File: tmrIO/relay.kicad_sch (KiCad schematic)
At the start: 5 parts, among them J1 Screw_Terminal_01x03, K1 Relay_SPDT, Q1 MMBT3904

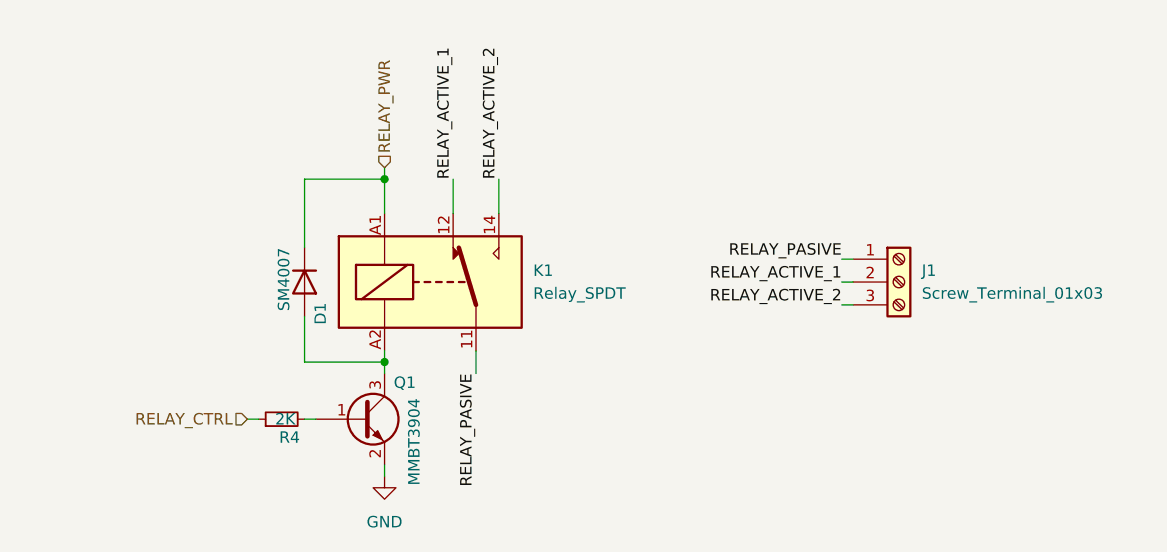
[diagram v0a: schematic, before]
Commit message: tmrIO update
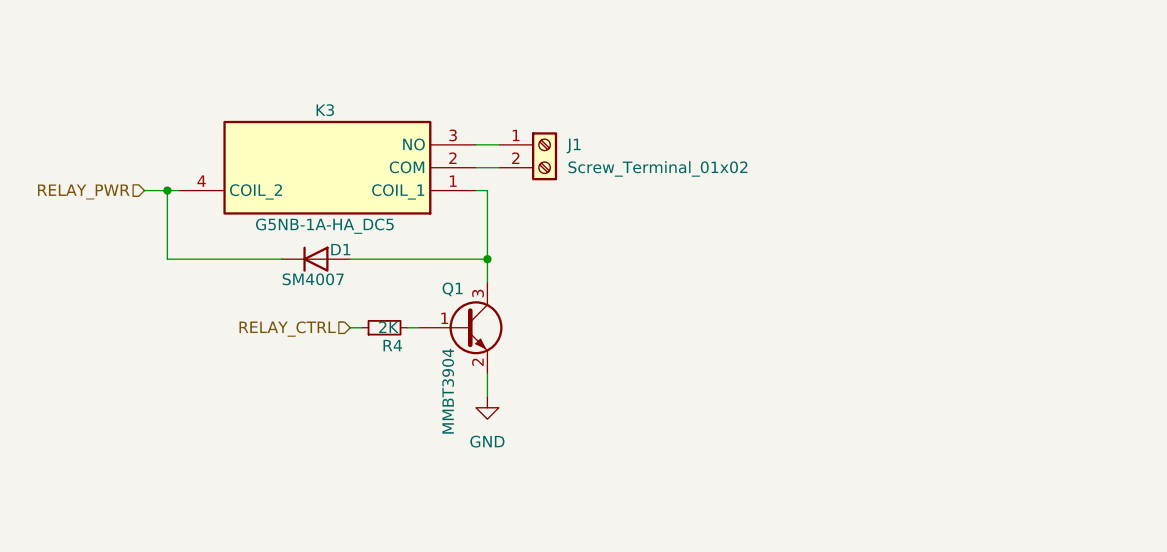
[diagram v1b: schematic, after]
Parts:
- removed J1: Screw_Terminal_01x03, symbol Connector:Screw_Terminal_01x03
- removed K1: Relay_SPDT, symbol Relay:Relay_SPDT
- added J1: Screw_Terminal_01x02, TerminalBlock_Phoenix:TerminalBlock_Phoenix_PT-1,5-2-3.5-H_1x02_P3.50mm_Horizontal, symbol Connector:Screw_Terminal_01x02
- added K3: G5NB-1A-HA_DC5, G5NB-1A-HA:G5NB1AHADC5, symbol G5NB-1A-HA_DC5:G5NB-1A-HA_DC5
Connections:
- net RELAY_PWR: now also K3.4 (COIL_2)
- net at D1.2 (A), Q1.3 (C): now also K3.1 (COIL_1)
- new net: J1.1 (Pin_1), K3.3 (NO)
- new net: J1.2 (Pin_2), K3.2 (COM)
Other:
- moved on the sheet: D1, Q1, R4
